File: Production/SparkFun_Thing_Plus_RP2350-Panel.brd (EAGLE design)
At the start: 83.3 x 80.3 mm, 486 parts, among them J1 THING_PLUS_LOGICAL, J12 MICRO-SD-ATOM, J13 THING_PLUS_LOGICAL, J15 QWIIC_RIGHT_ANGLE, J18 MICRO-SD-ATOM, J3 QWIIC_RIGHT_ANGLE, J6 MICRO-SD-ATOM, J7 THING_PLUS_LOGICAL, J9 QWIIC_RIGHT_ANGLE, Q1 100mA/20V/3.8Ω, Q2 100mA/20V/3.8Ω, Q3 100mA/20V/3.8Ω, U1 RP2350A, U10 ESD Diode, U11 RP2350A, U12 RM2, U13 RT9080-33GJ5, U14 LM66200, U15 W25QXX128MBIT, U16 MCP73831, U17 WS2812_2020, U18 MAX17048, U19 RT9080-33GJ5, U2 RM2, U20 ESD Diode, U21 RP2350A, U22 RM2, U23 RT9080-33GJ5, U24 LM66200, U25 W25QXX128MBIT, U26 MCP73831, U27 WS2812_2020, U28 MAX17048, U29 RT9080-33GJ5, U3 RT9080-33GJ5, U30 ESD Diode, U4 LM66200, U5 W25QXX128MBIT, U6 MCP73831, U7 WS2812_2020, U8 MAX17048, U9 RT9080-33GJ5, Y1 12MHz, Y2 12MHz, Y3 12MHz

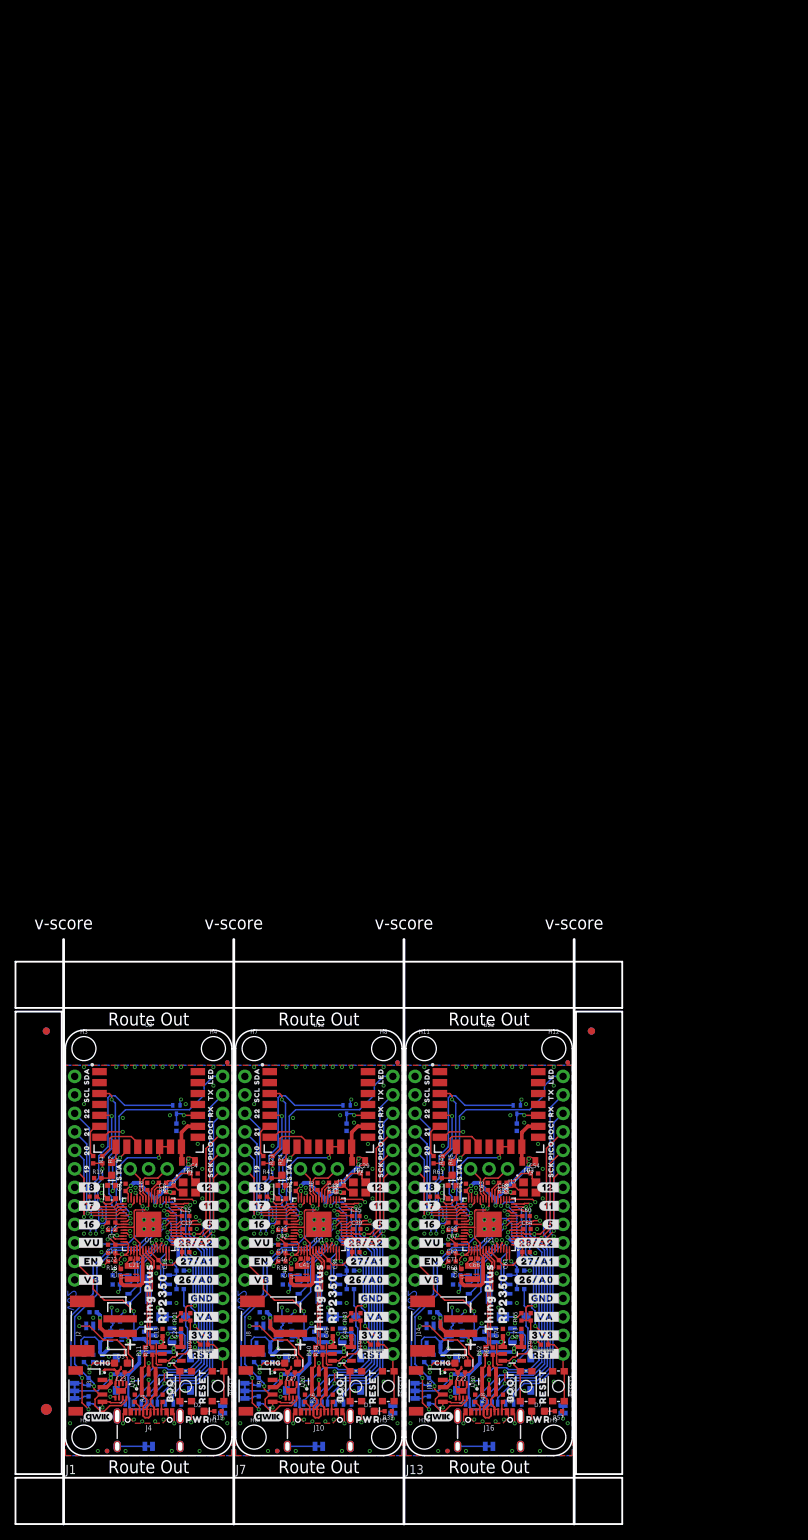
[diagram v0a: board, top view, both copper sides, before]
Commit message: Add v10 production files
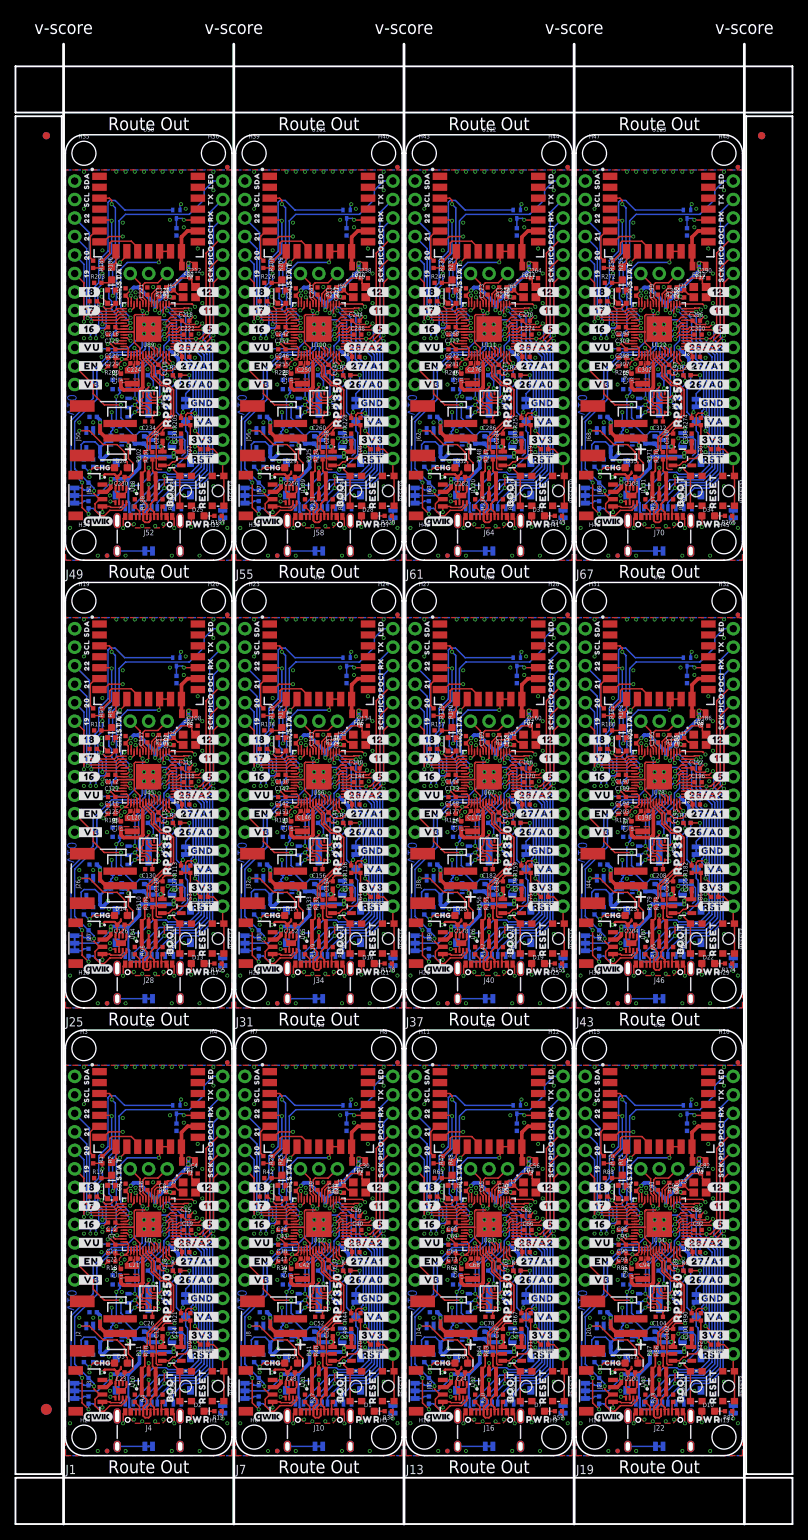
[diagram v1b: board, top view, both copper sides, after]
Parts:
- added BOOT10, BOOT11, BOOT3, BOOT4, BOOT5, BOOT6, BOOT7, BOOT8, BOOT9, RESET10, RESET11, RESET3, RESET4, RESET5, RESET6, RESET7, RESET8, RESET9: MOMENTARY-SWITCH-SPST-SMD-4.6X2.8MM, SparkFun-Switches:TACTILE_SWITCH_SMD_4.6X2.8MM
- added C100, C103, C104, C111, C112, C113, C114, C115, C116, C117, C118, C121, C122, C124, C126, C129, C130, C137, C138, C139, C140, C141, C142, C143, C144, C147, C148, C150, C152, C155, C156, C163, C164, C165, C166, C167, C168, C169, C170, C173, C174, C176, C178, C181, C182, C189, C190, C191, C192, C193, C194, C195, C196, C199, C200, C202, C204, C207, C208, C215, C216, C217, C218, C219, C220, C221, C222, C225, C226, C228, C230, C233, C234, C241, C242, C243, C244, C245, C246, C247, C248, C251, C252, C254, C256, C259, C260, C267, C268, C269, C270, C271, C272, C273, C274, C277, C278, C280, C282, C285, C286, C293, C294, C295, C296, C297, C298, C299, C300, C303, C304, C306, C308, C311, C312, C77, C78, C85, C86, C87, C88, C89, C90, C91, C92, C95, C96, C98: 0.1uF, SparkFun-Capacitors:0402-TIGHT
- added C101, C119, C120, C127, C145, C146, C153, C171, C172, C179, C197, C198, C205, C223, C224, C231, C249, C250, C257, C275, C276, C283, C301, C302, C309, C93, C94: 10uF, SparkFun-Capacitors:0402-TIGHT
- added C102, C105, C106, C109, C110, C123, C125, C128, C131, C132, C135, C136, C149, C151, C154, C157, C158, C161, C162, C175, C177, C180, C183, C184, C187, C188, C201, C203, C206, C209, C210, C213, C214, C227, C229, C232, C235, C236, C239, C240, C253, C255, C258, C261, C262, C265, C266, C279, C281, C284, C287, C288, C291, C292, C305, C307, C310, C76, C79, C80, C83, C84, C97, C99: 2.2uF, SparkFun-Capacitors:0402-TIGHT
- added C107, C108, C133, C134, C159, C160, C185, C186, C211, C212, C237, C238, C263, C264, C289, C290, C81, C82: 15pF, SparkFun-Capacitors:0402-TIGHT
- added D10, D13, D16, D19, D22, D25, D28, D31, D34: Red, SparkFun-LED:LED-0603
- added D11, D14, D17, D20, D23, D26, D29, D32, D35: Yellow, SparkFun-LED:LED-0603
- added D12, D15, D18, D21, D24, D27, D30, D33, D36: Blue, SparkFun-LED:LED-0603
- added FB10, FB11, FB12, FB4, FB5, FB6, FB7, FB8, FB9: 600Ω, SparkFun-Coils:0805
- added FD13, FD14, FD15, FD16, FD17, FD18, FD19, FD20, FD21, FD22, FD23, FD24, FD25, FD26, FD27, FD28, FD29, FD30, FD31, FD32, FD33, FD34, FD35, FD36, FD37, FD38, FD39, FD40, FD41, FD42, FD43, FD44, FD45, FD46, FD47, FD48: FIDUCIALUFIDUCIAL, SparkFun-Aesthetics:FIDUCIAL-MICRO
- added H13, H14, H15, H16, H17, H18, H19, H20, H21, H22, H23, H24, H25, H26, H27, H28, H29, H30, H31, H32, H33, H34, H35, H36, H37, H38, H39, H40, H41, H42, H43, H44, H45, H46, H47, H48: STAND-OFF, SparkFun-Hardware:STAND-OFF
- added I2C10, I2C11, I2C3, I2C4, I2C5, I2C6, I2C7, I2C8, I2C9: JUMPER-SMT_3_2-NC_TRACE_SILK, SparkFun-Jumpers:SMT-JUMPER_3_2-NC_TRACE_SILK
- added J19, J25, J31, J37, J43, J49, J55, J61, J67: THING_PLUS_LOGICAL, SparkFun-Boards:THING_PLUS
- added J20, J26, J32, J38, J44, J50, J56, J62, J68: (no value), SparkFun-Connectors:JST-2-SMD
- added J21, J27, J33, J39, J45, J51, J57, J63, J69: QWIIC_RIGHT_ANGLE, SparkFun-Connectors:JST04_1MM_RA
- added J22, J28, J34, J40, J46, J52, J58, J64, J70: (no value), SparkFun-Connectors:USB-C-16P_4LAYER-PADS
- added J23, J29, J35, J41, J47, J53, J59, J65, J71: (no value), SparkFun-Connectors:1X03_NO_SILK
- added J24, J30, J36, J42, J48, J54, J60, J66, J72: MICRO-SD-ATOM, SparkFun-Connectors:MICROSD_ATOM
- added L10, L11, L12, L4, L5, L6, L7, L8, L9: 4.7μH, SparkFun-Coils:1008(2520)
- added LOGO10, LOGO13, LOGO16, LOGO19, LOGO22, LOGO25, LOGO28, LOGO31, LOGO34: SFE_LOGO_NAME_FLAME.1_INCH, SparkFun-Aesthetics:SFE_LOGO_NAME_FLAME_.1
- added LOGO11, LOGO14, LOGO17, LOGO20, LOGO23, LOGO26, LOGO29, LOGO32, LOGO35: OSHW-LOGOS, SparkFun-Aesthetics:OSHW-LOGO-S
- added LOGO12, LOGO15, LOGO18, LOGO21, LOGO24, LOGO27, LOGO30, LOGO33, LOGO36: QWIIC_LOGO_4MM, SparkFun-Aesthetics:QWIIC_4MM
- added LP10, LP11, LP3, LP4, LP5, LP6, LP7, LP8, LP9, PWR10, PWR11, PWR3, PWR4, PWR5, PWR6, PWR7, PWR8, PWR9, SHLD10, SHLD11, SHLD3, SHLD4, SHLD5, SHLD6, SHLD7, SHLD8, SHLD9: JUMPER-SMT_2_NC_TRACE_SILK, SparkFun-Jumpers:SMT-JUMPER_2_NC_TRACE_SILK
- added Q10, Q11, Q12, Q4, Q5, Q6, Q7, Q8, Q9: 100mA/20V/3.8Ω, SparkFun-DiscreteSemi:SOT-416FL
- added R100, R102, R103, R112, R113, R115, R117, R123, R125, R126, R135, R136, R138, R140, R146, R148, R149, R158, R159, R161, R163, R169, R171, R172, R181, R182, R184, R186, R192, R194, R195, R204, R205, R207, R209, R215, R217, R218, R227, R228, R230, R232, R238, R240, R241, R250, R251, R253, R255, R261, R263, R264, R273, R274, R276, R67, R69, R71, R77, R79, R80, R89, R90, R92, R94: 10k, SparkFun-Resistors:0402-TIGHT
- added R101, R104, R124, R127, R147, R150, R170, R173, R193, R196, R216, R219, R239, R242, R262, R265, R78, R81: 1k, SparkFun-Resistors:0402-TIGHT
- added R105, R107, R128, R130, R151, R153, R174, R176, R197, R199, R220, R222, R243, R245, R266, R268, R82, R84: 4.7k, SparkFun-Resistors:0402-TIGHT
- added R106, R111, R120, R121, R129, R134, R143, R144, R152, R157, R166, R167, R175, R180, R189, R190, R198, R203, R212, R213, R221, R226, R235, R236, R244, R249, R258, R259, R267, R272, R74, R75, R83, R88, R97, R98: 2.2k, SparkFun-Resistors:0402-TIGHT
- added R108, R131, R154, R177, R200, R223, R246, R269, R85: 10Ω, SparkFun-Resistors:0402-TIGHT
- added R109, R110, R132, R133, R155, R156, R178, R179, R201, R202, R224, R225, R247, R248, R270, R271, R86, R87: 27OHM, SparkFun-Resistors:0402-TIGHT
- added R114, R122, R137, R145, R160, R168, R183, R191, R206, R214, R229, R237, R252, R260, R275, R68, R76, R91, R99: 1M, SparkFun-Resistors:0402-TIGHT
- added R116, R139, R162, R185, R208, R231, R254, R70, R93: 470, SparkFun-Resistors:0402-TIGHT
- added R118, R119, R141, R142, R164, R165, R187, R188, R210, R211, R233, R234, R256, R257, R72, R73, R95, R96: 5.1k, SparkFun-Resistors:0402-TIGHT
- added TP10, TP11, TP12, TP4, TP5, TP6, TP7, TP8, TP9: TEST-POINT3X5, SparkFun-Connectors:PAD.03X.05
- added U$217, U$288, U$359, U$430, U$501, U$572, U$643, U$714, U$785: (no value), output:RX0
- added U$218, U$289, U$360, U$431, U$502, U$573, U$644, U$715, U$786: (no value), output:PICO0
- added U$219, U$290, U$361, U$432, U$503, U$574, U$645, U$716, U$787: (no value), output:POCI0
- added U$220, U$291, U$362, U$433, U$504, U$575, U$646, U$717, U$788: (no value), output:SCK0
- added U$221, U$292, U$363, U$434, U$505, U$576, U$647, U$718, U$789: (no value), output:#SDA_#0
- added U$222, U$293, U$364, U$435, U$506, U$577, U$648, U$719, U$790: (no value), output:#SCL_#0
- added U$223, U$294, U$365, U$436, U$507, U$578, U$649, U$720, U$791: (no value), output:#_TX#0
- added U$224, U$295, U$366, U$437, U$508, U$579, U$650, U$721, U$792: (no value), output:#_RX#0
- added U$225, U$296, U$367, U$438, U$509, U$580, U$651, U$722, U$793: (no value), output:#_POCI#0
- added U$226, U$297, U$368, U$439, U$510, U$581, U$652, U$723, U$794: (no value), output:#_PICO#0
- added U$227, U$298, U$369, U$440, U$511, U$582, U$653, U$724, U$795: (no value), output:#_SCK#0
- added U$228, U$299, U$370, U$441, U$512, U$583, U$654, U$725, U$796: (no value), output:#_GND#0
- added U$229, U$300, U$371, U$442, U$513, U$584, U$655, U$726, U$797: (no value), output:#_3V3#0
- added U$230, U$301, U$372, U$443, U$514, U$585, U$656, U$727, U$798: (no value), output:#_SWCLK#0
- added U$231, U$302, U$373, U$444, U$515, U$586, U$657, U$728, U$799: (no value), output:#_SWDIO#0
- added U$232, U$303, U$374, U$445, U$516, U$587, U$658, U$729, U$800: (no value), output:#_VB#0
- added U$233, U$304, U$375, U$446, U$517, U$588, U$659, U$730, U$801: (no value), output:#_VU#0
- added U$234, U$305, U$376, U$447, U$518, U$589, U$660, U$731, U$802: (no value), output:#_EN#0
- added U$235, U$306, U$377, U$448, U$519, U$590, U$661, U$732, U$803: (no value), output:#3V3_#0
- added U$236, U$307, U$378, U$449, U$520, U$591, U$662, U$733, U$804: (no value), output:#GND_#0
- added U$237, U$308, U$379, U$450, U$521, U$592, U$663, U$734, U$805: (no value), output:#26#A0_#0
- added U$238, U$309, U$380, U$451, U$522, U$593, U$664, U$735, U$806: (no value), output:#27#A1_#0
- added U$239, U$310, U$381, U$452, U$523, U$594, U$665, U$736, U$807: (no value), output:#28#A2_#0
- added U$240, U$311, U$382, U$453, U$524, U$595, U$666, U$737, U$808: (no value), output:BOOT0
- added U$241, U$312, U$383, U$454, U$525, U$596, U$667, U$738, U$809: (no value), output:RESET0
- added U$242, U$313, U$384, U$455, U$526, U$597, U$668, U$739, U$810: (no value), output:#VU_#0
- added U$243, U$314, U$385, U$456, U$527, U$598, U$669, U$740, U$811: (no value), output:#VB_#0
- added U$244, U$315, U$386, U$457, U$528, U$599, U$670, U$741, U$812: (no value), output:#EN_#0
- added U$245, U$316, U$387, U$458, U$529, U$600, U$671, U$742, U$813: (no value), output:#_A1#27#0
- added U$246, U$317, U$388, U$459, U$530, U$601, U$672, U$743, U$814: (no value), output:#_A2#28#0
- added U$247, U$318, U$389, U$460, U$531, U$602, U$673, U$744, U$815: (no value), output:#I2C#0
- added U$248, U$319, U$390, U$461, U$532, U$603, U$674, U$745, U$816: (no value), output:#SHLD#0
- added U$249, U$320, U$391, U$462, U$533, U$604, U$675, U$746, U$817: (no value), output:THING_PLUS0
- added U$250, U$251, U$321, U$322, U$392, U$393, U$463, U$464, U$534, U$535, U$605, U$606, U$676, U$677, U$747, U$748, U$818, U$819: (no value), output:RP23500
- added U$252, U$323, U$394, U$465, U$536, U$607, U$678, U$749, U$820: (no value), output:#_16#0
- added U$253, U$324, U$395, U$466, U$537, U$608, U$679, U$750, U$821: (no value), output:#_17#0
- added U$254, U$325, U$396, U$467, U$538, U$609, U$680, U$751, U$822: (no value), output:#_18#0
- added U$255, U$326, U$397, U$468, U$539, U$610, U$681, U$752, U$823: (no value), output:200
- added U$256, U$327, U$398, U$469, U$540, U$611, U$682, U$753, U$824: (no value), output:210
- added U$257, U$328, U$399, U$470, U$541, U$612, U$683, U$754, U$825: (no value), output:220
- added U$258, U$329, U$400, U$471, U$542, U$613, U$684, U$755, U$826: (no value), output:#22_#0
- added U$259, U$330, U$401, U$472, U$543, U$614, U$685, U$756, U$827: (no value), output:#21_#0
- added U$260, U$331, U$402, U$473, U$544, U$615, U$686, U$757, U$828: (no value), output:#20_#0
- added U$261, U$332, U$403, U$474, U$545, U$616, U$687, U$758, U$829: (no value), output:#19_#0
- added U$262, U$333, U$404, U$475, U$546, U$617, U$688, U$759, U$830: (no value), output:#18_#0
- added U$263, U$334, U$405, U$476, U$547, U$618, U$689, U$760, U$831: (no value), output:#17_#0
- added U$264, U$335, U$406, U$477, U$548, U$619, U$690, U$761, U$832: (no value), output:#16_#0
- added U$265, U$336, U$407, U$478, U$549, U$620, U$691, U$762, U$833: (no value), output:190
- added U$266, U$337, U$408, U$479, U$550, U$621, U$692, U$763, U$834: (no value), output:CHG0
- added U$267, U$277, U$338, U$348, U$409, U$419, U$480, U$490, U$551, U$561, U$622, U$632, U$693, U$703, U$764, U$774, U$835, U$845: (no value), output:##RST#_#0
- added U$268, U$339, U$410, U$481, U$552, U$623, U$694, U$765, U$836: (no value), output:#PWR#0
- added U$269, U$340, U$411, U$482, U$553, U$624, U$695, U$766, U$837: (no value), output:PWR0
- added U$270, U$341, U$412, U$483, U$554, U$625, U$696, U$767, U$838: (no value), output:STAT0
- added U$271, U$342, U$413, U$484, U$555, U$626, U$697, U$768, U$839: (no value), output:#5_#0
- added U$272, U$343, U$414, U$485, U$556, U$627, U$698, U$769, U$840: (no value), output:LED0
- added U$273, U$344, U$415, U$486, U$557, U$628, U$699, U$770, U$841: (no value), output:#_LED#0
- added U$274, U$345, U$416, U$487, U$558, U$629, U$700, U$771, U$842: (no value), output:#_5#0
- added U$275, U$346, U$417, U$488, U$559, U$630, U$701, U$772, U$843: (no value), output:#VA_#0
- added U$276, U$347, U$418, U$489, U$560, U$631, U$702, U$773, U$844: (no value), output:#_VA#0
- added U$278, U$349, U$420, U$491, U$562, U$633, U$704, U$775, U$846: (no value), output:#LP#0
- added U$279, U$350, U$421, U$492, U$563, U$634, U$705, U$776, U$847: (no value), output:#11_#0
- added U$280, U$351, U$422, U$493, U$564, U$635, U$706, U$777, U$848: (no value), output:#12_#0
- added U$281, U$352, U$423, U$494, U$565, U$636, U$707, U$778, U$849: (no value), output:#_12#0
- added U$282, U$353, U$424, U$495, U$566, U$637, U$708, U$779, U$850: (no value), output:#_11#0
- added U$283, U$354, U$425, U$496, U$567, U$638, U$709, U$780, U$851: (no value), output:#_G#0
- added U$284, U$355, U$426, U$497, U$568, U$639, U$710, U$781, U$852: (no value), output:#_A0#0
- added U$285, U$356, U$427, U$498, U$569, U$640, U$711, U$782: (no value), output:SDA0
- added U$286, U$357, U$428, U$499, U$570, U$641, U$712, U$783: (no value), output:SCL0
- added U$287, U$358, U$429, U$500, U$571, U$642, U$713, U$784: (no value), output:TX0
- added U100, U111, U122, U34, U45, U56, U67, U78, U89: RP2350A, RP2350A:RP2350A
- added U101, U112, U123, U35, U46, U57, U68, U79, U90: RM2, RM2:RM2
- added U102, U108, U113, U119, U124, U130, U31, U36, U42, U47, U53, U58, U64, U69, U75, U80, U86, U91, U97: RT9080-33GJ5, SparkFun-IC-Power:SOT23-5
- added U103, U114, U125, U37, U48, U59, U70, U81, U92: LM66200, SparkFun-IC-Power:SOT8
- added U104, U115, U126, U38, U49, U60, U71, U82, U93: W25QXX128MBIT, SparkFun-IC-Memory:WSON-8-6X5-SKINNY_CENTERPAD
- added U105, U116, U127, U39, U50, U61, U72, U83, U94: MCP73831, SparkFun-IC-Power:SOT23-5
- added U106, U117, U128, U40, U51, U62, U73, U84, U95: WS2812_2020, SparkFun-LED:WS2812-2020
- added U107, U118, U129, U41, U52, U63, U74, U85, U96: MAX17048, SparkFun-IC-Power:DFN-8
- added U109, U120, U131, U32, U43, U54, U65, U76, U87, U98: ESD Diode, SparkFun-DiscreteSemi:SOT-23-6
- added U110, U121, U132, U33, U44, U55, U66, U77, U88, U99: APS6404L-3SQR-ZR, RP2350A:APS6404L-3SQR-ZR
- added Y10, Y11, Y12, Y4, Y5, Y6, Y7, Y8, Y9: 12MHz, SparkFun-Clocks:CRYSTAL-SMD-2X2.5MM
- C26, C44, C46, C51, C52, C69, C74: value 2.2uF -> 0.1uF
- C28, C53, C54: value 15pF -> 2.2uF
- C30, C55, C56: value 2.2uF -> 15pF
- C32, C45, C47, C50, C57, C58: value 0.1uF -> 2.2uF
- C40, C48, C65, C66: value 10uF -> 0.1uF
- C42, C67, C68, C75: value 0.1uF -> 10uF
- C49: value 2.2uF -> 10uF
- C73: value 10uF -> 2.2uF
- R23: value 470 -> 10k
- R24: value 10k -> 470
- R25, R48: value 5.1k -> 10k
- R27, R49, R50: value 2.2k -> 5.1k
- R29, R51: value 1M -> 2.2k
- R30: value 10k -> 1M
- R31, R34, R56: value 1k -> 10k
- R32, R55: value 10k -> 1k
- R35: value 4.7k -> 1k
- R36: value 2.2k -> 4.7k
- R37: value 4.7k -> 2.2k
- R38: value 10Ω -> 4.7k
- R39, R62: value 27OHM -> 10Ω
- R41, R63: value 2.2k -> 27OHM
- R42, R52, R65: value 10k -> 2.2k
- R44, R66: value 1M -> 10k
- R45: value 470 -> 1M
- R47: value 5.1k -> 470
- R53: value 1k -> 1M
- R57: value 4.7k -> 10k
- R58: value 2.2k -> 1k
- R60: value 10Ω -> 2.2k
- R61: value 27OHM -> 4.7k
- R64: value 10k -> 27OHM
- U$100: device output:BOOT0 -> output:#VU_#0
- U$101: device output:RESET0 -> output:#VB_#0
- U$102: device output:#VU_#0 -> output:#EN_#0
- U$103: device output:#VB_#0 -> output:#_A1#27#0
- U$104: device output:#EN_#0 -> output:#_A2#28#0
- U$105: device output:#_A0#26#0 -> output:#I2C#0
- U$106: device output:#_A1#27#0 -> output:#SHLD#0
- U$107: device output:#_A2#28#0 -> output:THING_PLUS0
- U$108, U$180: device output:#I2C#0 -> output:RP23500
- U$109: device output:#SHLD#0 -> output:RP23500
- U$110: device output:THING_PLUS0 -> output:#_16#0
- U$111: device output:RP23500 -> output:#_17#0
- U$112: device output:THING_PLUS0 -> output:#_18#0
- U$113: device output:RP23500 -> output:200
- U$114: device output:#_16#0 -> output:210
- U$115: device output:#_17#0 -> output:220
- U$116: device output:#_18#0 -> output:#22_#0
- U$117: device output:200 -> output:#21_#0
- U$118: device output:210 -> output:#20_#0
- U$119: device output:220 -> output:#19_#0
- U$120: device output:#22_#0 -> output:#18_#0
- U$121: device output:#21_#0 -> output:#17_#0
- U$122: device output:#20_#0 -> output:#16_#0
- U$123: device output:#19_#0 -> output:190
- U$124: device output:#18_#0 -> output:CHG0
- U$125: device output:#17_#0 -> output:##RST#_#0
- U$126: device output:#16_#0 -> output:#PWR#0
- U$127: device output:190 -> output:PWR0
- U$128: device output:CHG0 -> output:STAT0
- U$129: device output:##RST#_#0 -> output:#5_#0
- U$130: device output:#PWR#0 -> output:LED0
- U$131: device output:PWR0 -> output:#_LED#0
- U$132: device output:STAT0 -> output:#_5#0
- U$133: device output:#5_#0 -> output:#VA_#0
- U$134: device output:LED0 -> output:#_VA#0
- U$135: device output:#_LED#0 -> output:##RST#_#0
- U$136: device output:#_5#0 -> output:#LP#0
- U$137: device output:#VA_#0 -> output:#11_#0
- U$138: device output:#_VA#0 -> output:#12_#0
- U$139: device output:##RST#_#0 -> output:#_12#0
- U$140: device output:#LP#0 -> output:#_11#0
- U$141: device output:#11_#0 -> output:#_G#0
- U$142: device output:#12_#0 -> output:#_A0#0
- U$143: device output:#_12#0 -> output:SDA0
- U$144: device output:#_11#0 -> output:SCL0
- U$145: device output:SDA0 -> output:TX0
- U$146: device output:SCL0 -> output:RX0
- U$147: device output:TX0 -> output:PICO0
- U$148: device output:RX0 -> output:POCI0
- U$149: device output:PICO0 -> output:SCK0
- U$150: device output:POCI0 -> output:#SDA_#0
- U$151: device output:SCK0 -> output:#SCL_#0
- U$152: device output:#SDA_#0 -> output:#_TX#0
- U$153: device output:#SCL_#0 -> output:#_RX#0
- U$154: device output:#_TX#0 -> output:#_POCI#0
- U$155: device output:#_RX#0 -> output:#_PICO#0
- U$156: device output:#_POCI#0 -> output:#_SCK#0
- U$157: device output:#_PICO#0 -> output:#_GND#0
- U$158: device output:#_SCK#0 -> output:#_3V3#0
- U$159, U$88: device output:#_GND#0 -> output:#_SWCLK#0
- U$16: device output:#_GND#0 -> output:#_A0#0
- U$160: device output:#_GND#0 -> output:#_SWDIO#0
- U$161: device output:#_3V3#0 -> output:#_VB#0
- U$162: device output:#_SWCLK#0 -> output:#_VU#0
- U$163: device output:#_SWDIO#0 -> output:#_EN#0
- U$164: device output:#_VB#0 -> output:#3V3_#0
- U$165: device output:#_VU#0 -> output:#GND_#0
- U$166: device output:#_EN#0 -> output:#26#A0_#0
- U$167: device output:#3V3_#0 -> output:#27#A1_#0
- U$168: device output:#GND_#0 -> output:#28#A2_#0
- U$169: device output:#26#A0_#0 -> output:BOOT0
- U$170: device output:#27#A1_#0 -> output:RESET0
- U$171: device output:#28#A2_#0 -> output:#VU_#0
- U$172: device output:BOOT0 -> output:#VB_#0
- U$173: device output:RESET0 -> output:#EN_#0
- U$174: device output:#VU_#0 -> output:#_A1#27#0
- U$175: device output:#VB_#0 -> output:#_A2#28#0
- U$176: device output:#EN_#0 -> output:#I2C#0
- U$177: device output:#_A0#26#0 -> output:#SHLD#0
- U$178: device output:#_A1#27#0 -> output:THING_PLUS0
- U$179: device output:#_A2#28#0 -> output:RP23500
- U$181: device output:#SHLD#0 -> output:#_16#0
- U$182: device output:THING_PLUS0 -> output:#_17#0
- U$183: device output:RP23500 -> output:#_18#0
- U$184: device output:THING_PLUS0 -> output:200
- U$185: device output:RP23500 -> output:210
- U$186: device output:#_16#0 -> output:220
- U$187: device output:#_17#0 -> output:#22_#0
- U$188: device output:#_18#0 -> output:#21_#0
- U$189: device output:200 -> output:#20_#0
- U$190: device output:210 -> output:#19_#0
- U$191: device output:220 -> output:#18_#0
- U$192: device output:#22_#0 -> output:#17_#0
- U$193: device output:#21_#0 -> output:#16_#0
- U$194: device output:#20_#0 -> output:190
- U$195: device output:#19_#0 -> output:CHG0
- U$196: device output:#18_#0 -> output:##RST#_#0
- U$197: device output:#17_#0 -> output:#PWR#0
- U$198: device output:#16_#0 -> output:PWR0
- U$199: device output:190 -> output:STAT0
- U$200: device output:CHG0 -> output:#5_#0
- U$201: device output:##RST#_#0 -> output:LED0
- U$202: device output:#PWR#0 -> output:#_LED#0
- U$203: device output:PWR0 -> output:#_5#0
- U$204: device output:STAT0 -> output:#VA_#0
- U$205: device output:#5_#0 -> output:#_VA#0
- U$206: device output:LED0 -> output:##RST#_#0
- U$207: device output:#_LED#0 -> output:#LP#0
- U$208: device output:#_5#0 -> output:#11_#0
- U$209: device output:#VA_#0 -> output:#12_#0
- U$210: device output:#_VA#0 -> output:#_12#0
- U$211: device output:##RST#_#0 -> output:#_11#0
- U$212: device output:#LP#0 -> output:#_G#0
- U$213: device output:#11_#0 -> output:#_A0#0
- U$214: device output:#12_#0 -> output:SDA0
- U$215: device output:#_12#0 -> output:SCL0
- U$216: device output:#_11#0 -> output:TX0
- U$37: device output:#_A0#26#0 -> output:SDA0
- U$44: device output:THING_PLUS0 -> output:#_G#0
- U$71: device output:SDA0 -> output:SCL0
- U$74: device output:SCL0 -> output:TX0
- U$75: device output:TX0 -> output:RX0
- U$76: device output:RX0 -> output:PICO0
- U$77: device output:PICO0 -> output:POCI0
- U$78: device output:POCI0 -> output:SCK0
- U$79: device output:SCK0 -> output:#SDA_#0
- U$80: device output:#SDA_#0 -> output:#SCL_#0
- U$81: device output:#SCL_#0 -> output:#_TX#0
- U$82: device output:#_TX#0 -> output:#_RX#0
- U$83: device output:#_RX#0 -> output:#_POCI#0
- U$84: device output:#_POCI#0 -> output:#_PICO#0
- U$85: device output:#_PICO#0 -> output:#_SCK#0
- U$86: device output:#_SCK#0 -> output:#_GND#0
- U$87: device output:#_GND#0 -> output:#_3V3#0
- U$89: device output:#_3V3#0 -> output:#_SWDIO#0
- U$90: device output:#_SWCLK#0 -> output:#_VB#0
- U$91: device output:#_SWDIO#0 -> output:#_VU#0
- U$92: device output:#_VB#0 -> output:#_EN#0
- U$93: device output:#_VU#0 -> output:#3V3_#0
- U$94: device output:#_EN#0 -> output:#GND_#0
- U$95: device output:#3V3_#0 -> output:#26#A0_#0
- U$96: device output:#GND_#0 -> output:#27#A1_#0
- U$97: device output:#26#A0_#0 -> output:#28#A2_#0
- U$98: device output:#27#A1_#0 -> output:BOOT0
- U$99: device output:#28#A2_#0 -> output:RESET0
- U11: value RP2350A -> APS6404L-3SQR-ZR; device RP2350A:RP2350A -> RP2350A:APS6404L-3SQR-ZR
- U12: value RM2 -> RP2350A; device RM2:RM2 -> RP2350A:RP2350A
- U13: value RT9080-33GJ5 -> RM2; device SparkFun-IC-Power:SOT23-5 -> RM2:RM2
- U14: value LM66200 -> RT9080-33GJ5; device SparkFun-IC-Power:SOT8 -> SparkFun-IC-Power:SOT23-5
- U15: value W25QXX128MBIT -> LM66200; device SparkFun-IC-Memory:WSON-8-6X5-SKINNY_CENTERPAD -> SparkFun-IC-Power:SOT8
- U16: value MCP73831 -> W25QXX128MBIT; device SparkFun-IC-Power:SOT23-5 -> SparkFun-IC-Memory:WSON-8-6X5-SKINNY_CENTERPAD
- U17: value WS2812_2020 -> MCP73831; device SparkFun-LED:WS2812-2020 -> SparkFun-IC-Power:SOT23-5
- U18: value MAX17048 -> WS2812_2020; device SparkFun-IC-Power:DFN-8 -> SparkFun-LED:WS2812-2020
- U19: value RT9080-33GJ5 -> MAX17048; device SparkFun-IC-Power:SOT23-5 -> SparkFun-IC-Power:DFN-8
- U20: value ESD Diode -> RT9080-33GJ5; device SparkFun-DiscreteSemi:SOT-23-6 -> SparkFun-IC-Power:SOT23-5
- U21: value RP2350A -> ESD Diode; device RP2350A:RP2350A -> SparkFun-DiscreteSemi:SOT-23-6
- U22: value RM2 -> APS6404L-3SQR-ZR; device RM2:RM2 -> RP2350A:APS6404L-3SQR-ZR
- U23: value RT9080-33GJ5 -> RP2350A; device SparkFun-IC-Power:SOT23-5 -> RP2350A:RP2350A
- U24: value LM66200 -> RM2; device SparkFun-IC-Power:SOT8 -> RM2:RM2
- U25: value W25QXX128MBIT -> RT9080-33GJ5; device SparkFun-IC-Memory:WSON-8-6X5-SKINNY_CENTERPAD -> SparkFun-IC-Power:SOT23-5
- U26: value MCP73831 -> LM66200; device SparkFun-IC-Power:SOT23-5 -> SparkFun-IC-Power:SOT8
- U27: value WS2812_2020 -> W25QXX128MBIT; device SparkFun-LED:WS2812-2020 -> SparkFun-IC-Memory:WSON-8-6X5-SKINNY_CENTERPAD
- U28: value MAX17048 -> MCP73831; device SparkFun-IC-Power:DFN-8 -> SparkFun-IC-Power:SOT23-5
- U29: value RT9080-33GJ5 -> WS2812_2020; device SparkFun-IC-Power:SOT23-5 -> SparkFun-LED:WS2812-2020
- U30: value ESD Diode -> MAX17048; device SparkFun-DiscreteSemi:SOT-23-6 -> SparkFun-IC-Power:DFN-8
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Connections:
- new net !BATT_ALERT!10: U111.19, U118.5
- new net !BATT_ALERT!11: U122.19, U129.5
- new net !BATT_ALERT!3: U34.19, U41.5
- new net !BATT_ALERT!4: U45.19, U52.5
- new net !BATT_ALERT!5: U56.19, U63.5
- new net !BATT_ALERT!6: U67.19, U74.5
- new net !BATT_ALERT!7: U78.19, U85.5
- new net !BATT_ALERT!8: U89.19, U96.5
- new net !BATT_ALERT!9: U100.19, U107.5
- new net !BOOT!10: BOOT10.3, BOOT10.4, R242.2, TP11.1
- new net !BOOT!11: BOOT11.3, BOOT11.4, R265.2, TP12.1
- new net !BOOT!3: BOOT3.3, BOOT3.4, R81.2, TP4.1
- new net !BOOT!4: BOOT4.3, BOOT4.4, R104.2, TP5.1
- new net !BOOT!5: BOOT5.3, BOOT5.4, R127.2, TP6.1
- new net !BOOT!6: BOOT6.3, BOOT6.4, R150.2, TP7.1
- new net !BOOT!7: BOOT7.3, BOOT7.4, R173.2, TP8.1
- new net !BOOT!8: BOOT8.3, BOOT8.4, R196.2, TP9.1
- new net !BOOT!9: BOOT9.3, BOOT9.4, R219.2, TP10.1
- new net !RESET!10: J61.28, R240.1, RESET10.3, RESET10.4, U111.26
- new net !RESET!11: J67.28, R263.1, RESET11.3, RESET11.4, U122.26
- new net !RESET!3: J19.28, R79.1, RESET3.3, RESET3.4, U34.26
- new net !RESET!4: J25.28, R102.1, RESET4.3, RESET4.4, U45.26
- new net !RESET!5: J31.28, R125.1, RESET5.3, RESET5.4, U56.26
- new net !RESET!6: J37.28, R148.1, RESET6.3, RESET6.4, U67.26
- new net !RESET!7: J43.28, R171.1, RESET7.3, RESET7.4, U78.26
- new net !RESET!8: J49.28, R194.1, RESET8.3, RESET8.4, U89.26
- new net !RESET!9: J55.28, R217.1, RESET9.3, RESET9.4, U100.26
- new net 1.1V10: C273.1, C274.1, C275.1, C277.1, L11.1, U111.23, U111.39, U111.50, U111.6
- new net 1.1V11: C299.1, C300.1, C301.1, C303.1, L12.1, U122.23, U122.39, U122.50, U122.6
- new net 1.1V3: C91.1, C92.1, C93.1, C95.1, L4.1, U34.23, U34.39, U34.50, U34.6
- new net 1.1V4: C117.1, C118.1, C119.1, C121.1, L5.1, U45.23, U45.39, U45.50, U45.6
- new net 1.1V5: C143.1, C144.1, C145.1, C147.1, L6.1, U56.23, U56.39, U56.50, U56.6
- new net 1.1V6: C169.1, C170.1, C171.1, C173.1, L7.1, U67.23, U67.39, U67.50, U67.6
- new net 1.1V7: C195.1, C196.1, C197.1, C199.1, L8.1, U78.23, U78.39, U78.50, U78.6
- new net 1.1V8: C221.1, C222.1, C223.1, C225.1, L9.1, U89.23, U89.39, U89.50, U89.6
- new net 1.1V9: C247.1, C248.1, C249.1, C251.1, L10.1, U100.23, U100.39, U100.50, U100.6
- new net 3.3V10: C262.1, C267.1, C268.1, C269.1, C270.1, C271.1, C272.1, C276.1, C278.1, C279.1, C280.1, C286.1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
- new net 3.3V11: C288.1, C293.1, C294.1, C295.1, C296.1, C297.1, C298.1, C302.1, C304.1, C305.1, C306.1, C312.1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
- new net 3.3V3: C104.1, C80.1, C85.1, C86.1, C87.1, C88.1, C89.1, C90.1, C94.1, C96.1, C97.1, C98.1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
- new net 3.3V4: C106.1, C111.1, C112.1, C113.1, C114.1, C115.1, C116.1, C120.1, C122.1, C123.1, C124.1, C130.1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
- new net 3.3V5: C132.1, C137.1, C138.1, C139.1, C140.1, C141.1, C142.1, C146.1, C148.1, C149.1, C150.1, C156.1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
- new net 3.3V6: C158.1, C163.1, C164.1, C165.1, C166.1, C167.1, C168.1, C172.1, C174.1, C175.1, C176.1, C182.1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
- new net 3.3V7: C184.1, C189.1, C190.1, C191.1, C192.1, C193.1, C194.1, C198.1, C200.1, C201.1, C202.1, C208.1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
- new net 3.3V8: C210.1, C215.1, C216.1, C217.1, C218.1, C219.1, C220.1, C224.1, C226.1, C227.1, C228.1, C234.1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
- new net 3.3V9: C236.1, C241.1, C242.1, C243.1, C244.1, C245.1, C246.1, C250.1, C252.1, C253.1, C254.1, C260.1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
- new net 3.3V_SW10: C283.1, C285.1, I2C10.2, J63.2, J66.4, U117.VCC, U119.5
- new net 3.3V_SW11: C309.1, C311.1, I2C11.2, J69.2, J72.4, U128.VCC, U130.5
- new net 3.3V_SW3: C101.1, C103.1, I2C3.2, J21.2, J24.4, U40.VCC, U42.5
- new net 3.3V_SW4: C127.1, C129.1, I2C4.2, J27.2, J30.4, U51.VCC, U53.5
- new net 3.3V_SW5: C153.1, C155.1, I2C5.2, J33.2, J36.4, U62.VCC, U64.5
- new net 3.3V_SW6: C179.1, C181.1, I2C6.2, J39.2, J42.4, U73.VCC, U75.5
- new net 3.3V_SW7: C205.1, C207.1, I2C7.2, J45.2, J48.4, U84.VCC, U86.5
- new net 3.3V_SW8: C231.1, C233.1, I2C8.2, J51.2, J54.4, U95.VCC, U97.5
- new net 3.3V_SW9: C257.1, C259.1, I2C9.2, J57.2, J60.4, U106.VCC, U108.5
- new net BAT_SW10: Q11.1, R238.1, U114.8
- new net BAT_SW11: Q12.1, R261.1, U125.8
- new net BAT_SW3: Q4.1, R77.1, U37.8
- new net BAT_SW4: Q5.1, R100.1, U48.8
- new net BAT_SW5: Q6.1, R123.1, U59.8
- new net BAT_SW6: Q7.1, R146.1, U70.8
- new net BAT_SW7: Q8.1, R169.1, U81.8
- new net BAT_SW8: Q9.1, R192.1, U92.8
- new net BAT_SW9: Q10.1, R215.1, U103.8
- new net EN10: J61.11, R237.2, U113.3
- new net EN11: J67.11, R260.2, U124.3
- new net EN3: J19.11, R76.2, U36.3
- new net EN4: J25.11, R99.2, U47.3
- new net EN5: J31.11, R122.2, U58.3
- new net EN6: J37.11, R145.2, U69.3
- new net EN7: J43.11, R168.2, U80.3
- new net EN8: J49.11, R191.2, U91.3
- new net EN9: J55.11, R214.2, U102.3
- new net GND10: BOOT10.1, BOOT10.2, C261.2, C262.2, C263.1, C264.2, C265.2, C266.2, C267.2, C268.2, C269.2, C270.2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
- new net GND11: BOOT11.1, BOOT11.2, C287.2, C288.2, C289.1, C290.2, C291.2, C292.2, C293.2, C294.2, C295.2, C296.2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
- new net GND3: BOOT3.1, BOOT3.2, C100.2, C101.2, C102.2, C103.2, C104.2, C79.2, C80.2, C81.1, C82.2, C83.2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
- new net GND4: BOOT4.1, BOOT4.2, C105.2, C106.2, C107.1, C108.2, C109.2, C110.2, C111.2, C112.2, C113.2, C114.2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
- new net GND5: BOOT5.1, BOOT5.2, C131.2, C132.2, C133.1, C134.2, C135.2, C136.2, C137.2, C138.2, C139.2, C140.2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
- new net GND6: BOOT6.1, BOOT6.2, C157.2, C158.2, C159.1, C160.2, C161.2, C162.2, C163.2, C164.2, C165.2, C166.2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
- new net GND7: BOOT7.1, BOOT7.2, C183.2, C184.2, C185.1, C186.2, C187.2, C188.2, C189.2, C190.2, C191.2, C192.2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
- new net GND8: BOOT8.1, BOOT8.2, C209.2, C210.2, C211.1, C212.2, C213.2, C214.2, C215.2, C216.2, C217.2, C218.2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
- new net GND9: BOOT9.1, BOOT9.2, C235.2, C236.2, C237.1, C238.2, C239.2, C240.2, C241.2, C242.2, C243.2, C244.2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
- new net GPIO100: J55.19, U100.16
- new net GPIO101: J61.3, U111.34
- new net GPIO102: J61.4, U111.33
- new net GPIO103: J61.5, U111.32
- new net GPIO104: J61.6, U111.31
- new net GPIO105: J61.7, U111.29
- new net GPIO106: J61.8, U111.28
- new net GPIO107: J61.9, U111.27
- new net GPIO108: J61.21, U111.8
- new net GPIO109: J61.20, U111.15
- new net GPIO110: J61.19, U111.16
- new net GPIO111: J67.3, U122.34
- new net GPIO112: J67.4, U122.33
- new net GPIO113: J67.5, U122.32
- new net GPIO114: J67.6, U122.31
- new net GPIO115: J67.7, U122.29
- new net GPIO116: J67.8, U122.28
- new net GPIO117: J67.9, U122.27
- new net GPIO118: J67.21, U122.8
- new net GPIO119: J67.20, U122.15
- new net GPIO120: J67.19, U122.16
- new net GPIO26/A10: J61.24, U111.40
- new net GPIO26/A11: J67.24, U122.40
- new net GPIO26/A3: J19.24, U34.40
- new net GPIO26/A4: J25.24, U45.40
- new net GPIO26/A5: J31.24, U56.40
- new net GPIO26/A6: J37.24, U67.40
- new net GPIO26/A7: J43.24, U78.40
- new net GPIO26/A8: J49.24, U89.40
- new net GPIO26/A9: J55.24, U100.40
- new net GPIO27/A10: J55.23, U100.41
- new net GPIO27/A11: J61.23, U111.41
- new net GPIO27/A12: J67.23, U122.41
- new net GPIO27/A4: J19.23, U34.41
- new net GPIO27/A5: J25.23, U45.41
- new net GPIO27/A6: J31.23, U56.41
- new net GPIO27/A7: J37.23, U67.41
- new net GPIO27/A8: J43.23, U78.41
- new net GPIO27/A9: J49.23, U89.41
- new net GPIO28/A10: J55.22, U100.42
- new net GPIO28/A11: J61.22, U111.42
- new net GPIO28/A12: J67.22, U122.42
- new net GPIO28/A4: J19.22, U34.42
- new net GPIO28/A5: J25.22, U45.42
- new net GPIO28/A6: J31.22, U56.42
- new net GPIO28/A7: J37.22, U67.42
- new net GPIO28/A8: J43.22, U78.42
- new net GPIO28/A9: J49.22, U89.42
- new net GPIO31: J19.3, U34.34
- new net GPIO32: J19.4, U34.33
- new net GPIO33: J19.5, U34.32
- new net GPIO34: J19.6, U34.31
- new net GPIO35: J19.7, U34.29
- new net GPIO36: J19.8, U34.28
- new net GPIO37: J19.9, U34.27
- new net GPIO38: J19.21, U34.8
- new net GPIO39: J19.20, U34.15
- new net GPIO40: J19.19, U34.16
- new net GPIO41: J25.3, U45.34
- new net GPIO42: J25.4, U45.33
- new net GPIO43: J25.5, U45.32
- new net GPIO44: J25.6, U45.31
- new net GPIO45: J25.7, U45.29
- new net GPIO46: J25.8, U45.28
- new net GPIO47: J25.9, U45.27
- new net GPIO48: J25.21, U45.8
- new net GPIO49: J25.20, U45.15
- new net GPIO50: J25.19, U45.16
- new net GPIO51: J31.3, U56.34
- new net GPIO52: J31.4, U56.33
- new net GPIO53: J31.5, U56.32
- new net GPIO54: J31.6, U56.31
- new net GPIO55: J31.7, U56.29
- new net GPIO56: J31.8, U56.28
- new net GPIO57: J31.9, U56.27
- new net GPIO58: J31.21, U56.8
- new net GPIO59: J31.20, U56.15
- new net GPIO60: J31.19, U56.16
- new net GPIO61: J37.3, U67.34
- new net GPIO62: J37.4, U67.33
- new net GPIO63: J37.5, U67.32
- new net GPIO64: J37.6, U67.31
- new net GPIO65: J37.7, U67.29
- new net GPIO66: J37.8, U67.28
- new net GPIO67: J37.9, U67.27
- new net GPIO68: J37.21, U67.8
- new net GPIO69: J37.20, U67.15
- new net GPIO70: J37.19, U67.16
- new net GPIO71: J43.3, U78.34
- new net GPIO72: J43.4, U78.33
- new net GPIO73: J43.5, U78.32
- new net GPIO74: J43.6, U78.31
- new net GPIO75: J43.7, U78.29
- new net GPIO76: J43.8, U78.28
- new net GPIO77: J43.9, U78.27
- new net GPIO78: J43.21, U78.8
- new net GPIO79: J43.20, U78.15
- new net GPIO80: J43.19, U78.16
- new net GPIO81: J49.3, U89.34
- new net GPIO82: J49.4, U89.33
- new net GPIO83: J49.5, U89.32
- new net GPIO84: J49.6, U89.31
- new net GPIO85: J49.7, U89.29
- new net GPIO86: J49.8, U89.28
- new net GPIO87: J49.9, U89.27
- new net GPIO88: J49.21, U89.8
- new net GPIO89: J49.20, U89.15
- new net GPIO90: J49.19, U89.16
- new net GPIO91: J55.3, U100.34
- new net GPIO92: J55.4, U100.33
- new net GPIO93: J55.5, U100.32
- new net GPIO94: J55.6, U100.31
- new net GPIO95: J55.7, U100.29
- new net GPIO96: J55.8, U100.28
- new net GPIO97: J55.9, U100.27
- new net GPIO98: J55.21, U100.8
- new net GPIO99: J55.20, U100.15
- new net LED_IN10: U111.18, U117.DI
- new net LED_IN11: U122.18, U128.DI
- new net LED_IN3: U34.18, U40.DI
- new net LED_IN4: U45.18, U51.DI
- new net LED_IN5: U56.18, U62.DI
- new net LED_IN6: U67.18, U73.DI
- new net LED_IN7: U78.18, U84.DI
- new net LED_IN8: U89.18, U95.DI
- new net LED_IN9: U100.18, U106.DI
- new net LED_OUT10: J61.13, U117.DO
- new net LED_OUT11: J67.13, U128.DO
- new net LED_OUT3: J19.13, U40.DO
- new net LED_OUT4: J25.13, U51.DO
- new net LED_OUT5: J31.13, U62.DO
- new net LED_OUT6: J37.13, U73.DO
- new net LED_OUT7: J43.13, U84.DO
- new net LED_OUT8: J49.13, U95.DO
- new net LED_OUT9: J55.13, U106.DO
- new net N$100: LP4.1, R113.2
- new net N$101: FB6.2, U57.B7, U57.C2
- new net N$102: R116.1, U57.A6
- new net N$103: R117.1, U57.B3
- new net N$104: J34.B5, R118.2
- new net N$105: J34.A5, R119.2
- new net N$106: J34.A7, J34.B7, R133.1, U65.1, U65.6
- new net N$107: J34.A6, J34.B6, R132.1, U65.3, U65.4
- new net N$108: I2C5.3, R120.2
- new net N$109: I2C5.1, R121.2
- new net N$110: C133.2, U56.21, Y6.P3
- new net N$111: C134.1, R124.1, Y6.P1
- new net N$112: R124.2, U56.22
- new net N$113: D16.C, R128.2
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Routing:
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- added copper zone on layer 1, net 1.1V10
- added copper zone on layer 1, net 1.1V11
- added copper zone on layer 1, net 1.1V3
- added copper zone on layer 1, net 1.1V4
- added copper zone on layer 1, net 1.1V5
- added copper zone on layer 1, net 1.1V6
- added copper zone on layer 1, net 1.1V7
- added copper zone on layer 1, net 1.1V8
- added copper zone on layer 1, net 1.1V9
- added copper zone on layer 1, net 3.3V10
- added copper zone on layer 15, net 3.3V10
- added copper zone on layer 16, net 3.3V10
- added copper zone on layer 1, net 3.3V11
- added copper zone on layer 15, net 3.3V11
- added copper zone on layer 16, net 3.3V11
- added copper zone on layer 1, net 3.3V3
- added copper zone on layer 15, net 3.3V3
- added copper zone on layer 16, net 3.3V3
- added copper zone on layer 1, net 3.3V4
- added copper zone on layer 15, net 3.3V4
- added copper zone on layer 16, net 3.3V4
- added copper zone on layer 1, net 3.3V5
- added copper zone on layer 15, net 3.3V5
- added copper zone on layer 16, net 3.3V5
- added copper zone on layer 1, net 3.3V6
- added copper zone on layer 15, net 3.3V6
- added copper zone on layer 16, net 3.3V6
- added copper zone on layer 1, net 3.3V7
- added copper zone on layer 15, net 3.3V7
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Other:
- board size 83.3 x 80.3 mm -> 106.7 x 203.2 mm
- board text added: "v10"
- board text removed: "v02"
